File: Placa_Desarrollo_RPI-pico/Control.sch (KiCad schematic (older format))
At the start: 0 parts

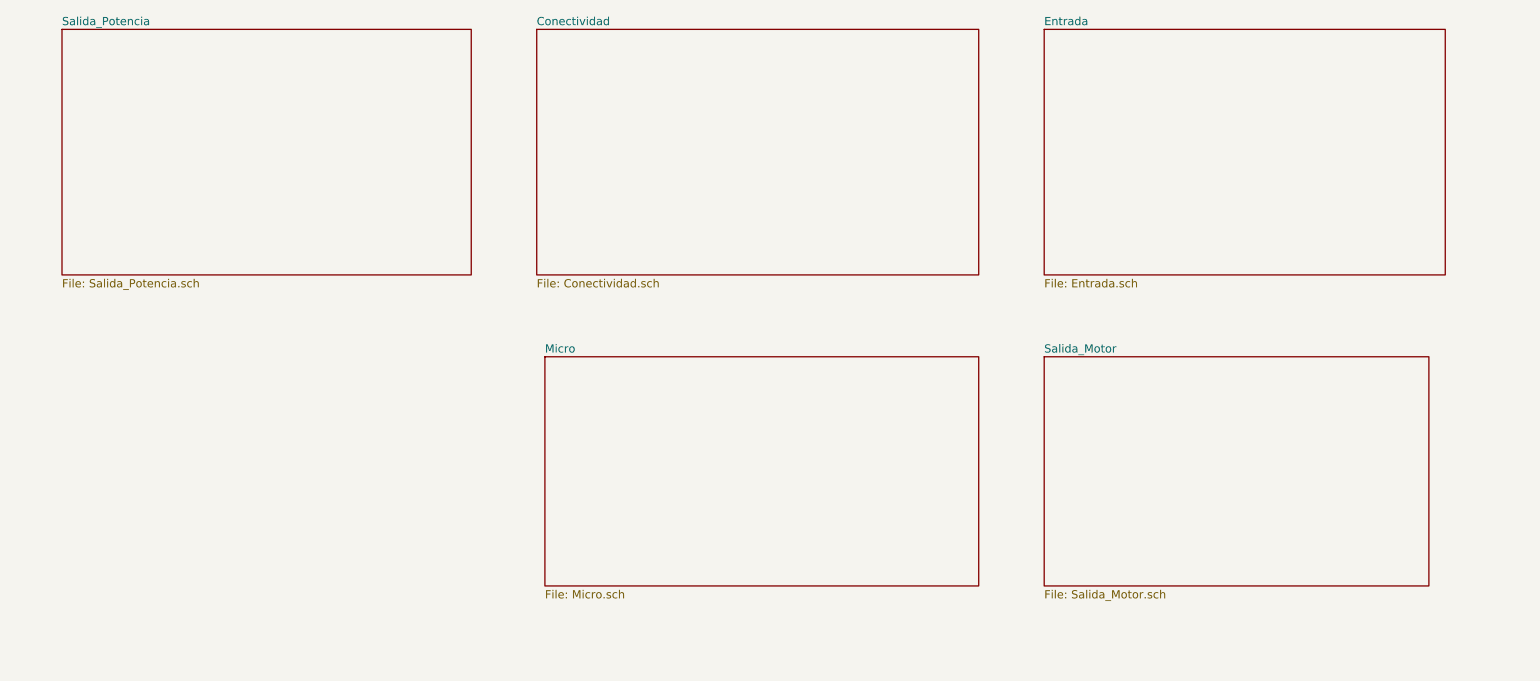
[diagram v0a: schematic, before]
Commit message: -
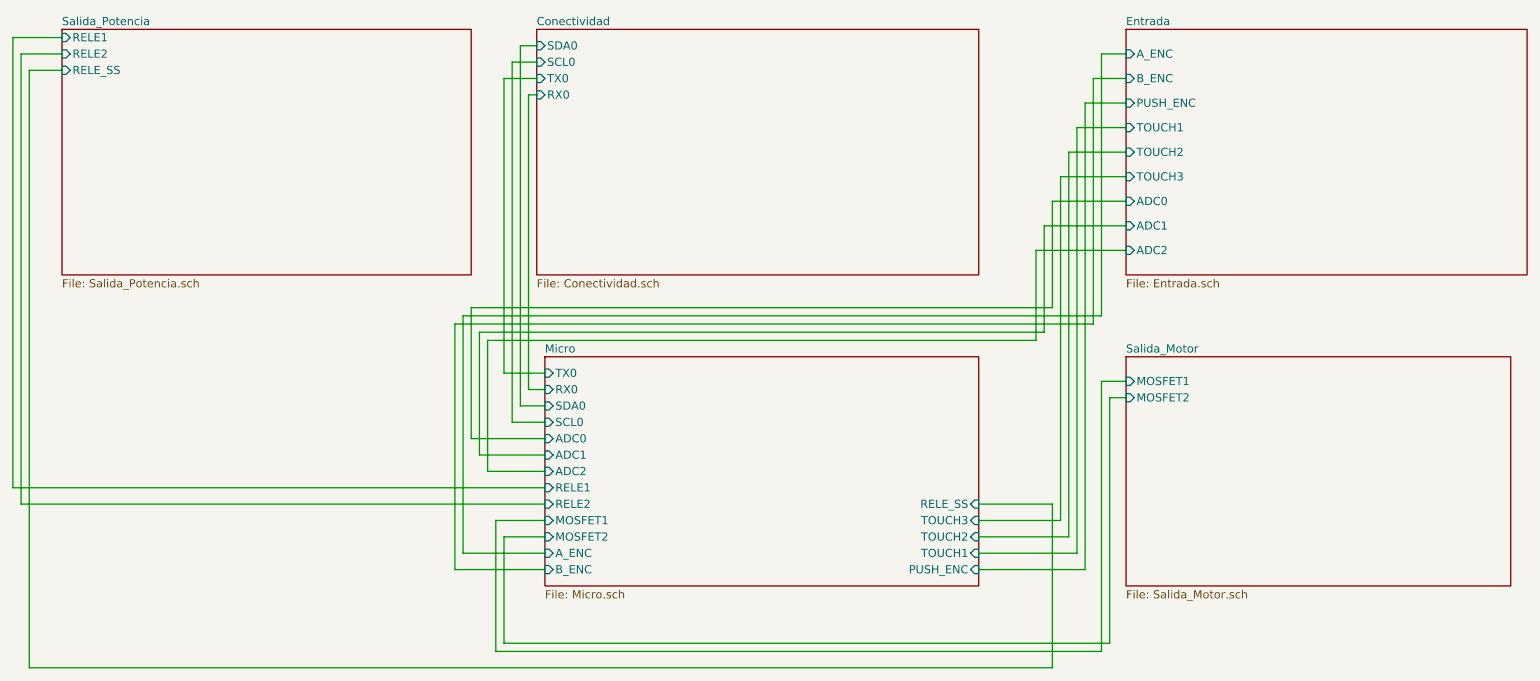
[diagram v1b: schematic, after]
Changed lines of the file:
@@
 F0 "Salida_Potencia" 50
 F1 "Salida_Potencia.sch" 50
+F2 "RELE1" I L 1050 1050 50
+F3 "RELE2" I L 1050 1150 50
+F4 "RELE_SS" I L 1050 1250 50
 $EndSheet
 $Sheet
@@
 F0 "Conectividad" 50
 F1 "Conectividad.sch" 50
-$EndSheet
-$Sheet
-S 7050 1000 2450 1500
+F2 "SDA0" I L 3950 1100 50
+F3 "SCL0" I L 3950 1200 50
+F4 "TX0" I L 3950 1300 50
+F5 "RX0" I L 3950 1400 50
+$EndSheet
+$Sheet
+S 7550 1000 2450 1500
 U 60B8603D
 F0 "Entrada" 50
 F1 "Entrada.sch" 50
-$EndSheet
-$Sheet
-S 7050 3000 2350 1400
+F2 "A_ENC" I L 7550 1150 50
+F3 "B_ENC" I L 7550 1300 50
+F4 "PUSH_ENC" I L 7550 1450 50
+F5 "TOUCH1" I L 7550 1600 50
+F6 "TOUCH2" I L 7550 1750 50
+F7 "TOUCH3" I L 7550 1900 50
+F8 "ADC0" I L 7550 2050 50
+F9 "ADC1" I L 7550 2200 50
+F10 "ADC2" I L 7550 2350 50
+$EndSheet
+$Sheet
+S 7550 3000 2350 1400
 U 60BE3D74
 F0 "Salida_Motor" 50
 F1 "Salida_Motor.sch" 50
+F2 "MOSFET1" I L 7550 3150 50
+F3 "MOSFET2" I L 7550 3250 50
 $EndSheet
 $Sheet
@@
 F0 "Micro" 50
 F1 "Micro.sch" 50
-$EndSheet
+F2 "TX0" I L 4000 3100 50
+F3 "RX0" I L 4000 3200 50
+F4 "SDA0" I L 4000 3300 50
+F5 "SCL0" I L 4000 3400 50
+F6 "ADC0" I L 4000 3500 50
+F7 "ADC1" I L 4000 3600 50
+F8 "ADC2" I L 4000 3700 50
+F9 "RELE1" I L 4000 3800 50
+F10 "RELE2" I L 4000 3900 50
+F11 "MOSFET1" I L 4000 4000 50
+F12 "MOSFET2" I L 4000 4100 50
+F13 "A_ENC" I L 4000 4200 50
+F14 "B_ENC" I L 4000 4300 50
+F15 "PUSH_ENC" I R 6650 4300 50
+F16 "TOUCH1" I R 6650 4200 50
+F17 "TOUCH2" I R 6650 4100 50
+F18 "TOUCH3" I R 6650 4000 50
+F19 "RELE_SS" I R 6650 3900 50
+$EndSheet
+Wire Wire Line
+	7550 3250 7450 3250
+Wire Wire Line
+	7450 3250 7450 4750
+Wire Wire Line
+	7450 4750 3750 4750
+Wire Wire Line
+	3750 4750 3750 4100
+Wire Wire Line
+	3750 4100 4000 4100
+Wire Wire Line
+	7550 3150 7400 3150
+Wire Wire Line
+	7400 3150 7400 4800
+Wire Wire Line
+	7400 4800 3700 4800
+Wire Wire Line
+	3700 4800 3700 4000
+Wire Wire Line
+	3700 4000 4000 4000
+Wire Wire Line
+	7550 1150 7400 1150
+Wire Wire Line
+	7400 1150 7400 2750
+Wire Wire Line
+	7400 2750 3500 2750
+Wire Wire Line
+	3500 2750 3500 4200
+Wire Wire Line
+	3500 4200 4000 4200
+Wire Wire Line
+	7550 1300 7350 1300
+Wire Wire Line
+	7350 1300 7350 2800
+Wire Wire Line
+	7350 2800 3450 2800
+Wire Wire Line
+	3450 2800 3450 4300
+Wire Wire Line
+	3450 4300 4000 4300
+Wire Wire Line
+	7550 1450 7300 1450
+Wire Wire Line
+	7300 1450 7300 4300
+Wire Wire Line
+	7300 4300 6650 4300
+Wire Wire Line
+	7550 1600 7250 1600
+Wire Wire Line
+	7250 1600 7250 4200
+Wire Wire Line
+	7250 4200 6650 4200
+Wire Wire Line
+	7550 1750 7200 1750
+Wire Wire Line
+	7200 1750 7200 4100
+Wire Wire Line
+	7200 4100 6650 4100
+Wire Wire Line
+	6650 4000 7150 4000
+Wire Wire Line
+	7150 4000 7150 1900
+Wire Wire Line
+	7150 1900 7550 1900
+Wire Wire Line
+	7550 2050 7100 2050
+Wire Wire Line
+	7100 2050 7100 2700
+Wire Wire Line
+	7100 2700 3550 2700
+Wire Wire Line
+	3550 2700 3550 3500
+Wire Wire Line
+	3550 3500 4000 3500
+Wire Wire Line
+	4000 3600 3600 3600
+Wire Wire Line
+	3600 3600 3600 2850
+Wire Wire Line
+	3600 2850 7050 2850
+Wire Wire Line
+	7050 2850 7050 2200
+Wire Wire Line
+	7050 2200 7550 2200
+Wire Wire Line
+	7550 2350 7000 2350
+Wire Wire Line
+	7000 2350 7000 2900
+Wire Wire Line
+	7000 2900 3650 2900
+Wire Wire Line
+	3650 2900 3650 3700
+Wire Wire Line
+	3650 3700 4000 3700
+Wire Wire Line
+	3950 1100 3850 1100
+Wire Wire Line
+	3850 1100 3850 3300
+Wire Wire Line
+	3850 3300 4000 3300
+Wire Wire Line
+	3950 1200 3800 1200
+Wire Wire Line
+	3800 1200 3800 3400
+Wire Wire Line
+	3800 3400 4000 3400
+Wire Wire Line
+	4000 3200 3900 3200
+Wire Wire Line
+	3900 3200 3900 1400
+Wire Wire Line
+	3900 1400 3950 1400
+Wire Wire Line
+	4000 3100 3750 3100
+Wire Wire Line
+	3750 3100 3750 1300
+Wire Wire Line
+	3750 1300 3950 1300
+Wire Wire Line
+	4000 3800 750  3800
+Wire Wire Line
+	750  3800 750  1050
+Wire Wire Line
+	750  1050 1050 1050
+Wire Wire Line
+	1050 1150 800  1150
+Wire Wire Line
+	800  1150 800  3900
+Wire Wire Line
+	800  3900 4000 3900
+Wire Wire Line
+	6650 3900 7100 3900
+Wire Wire Line
+	7100 3900 7100 4900
+Wire Wire Line
+	7100 4900 850  4900
+Wire Wire Line
+	850  4900 850  1250
+Wire Wire Line
+	850  1250 1050 1250
 $EndSCHEMATC
